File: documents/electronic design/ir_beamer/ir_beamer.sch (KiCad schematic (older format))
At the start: 10 parts, among them U1 74HC595D, U2 STM32F103HEADER

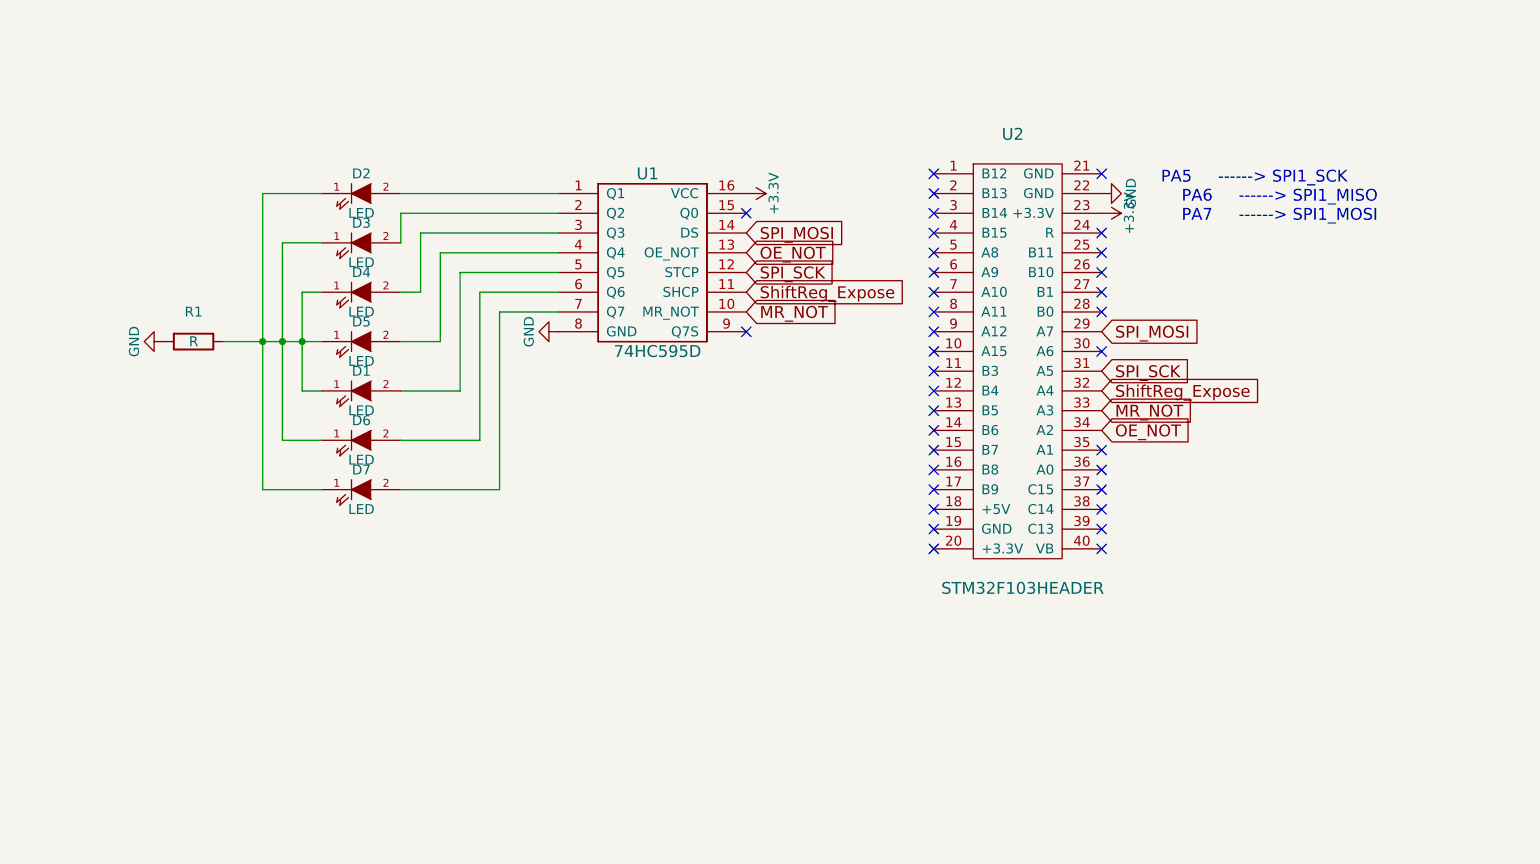
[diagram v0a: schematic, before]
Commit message: update pcb
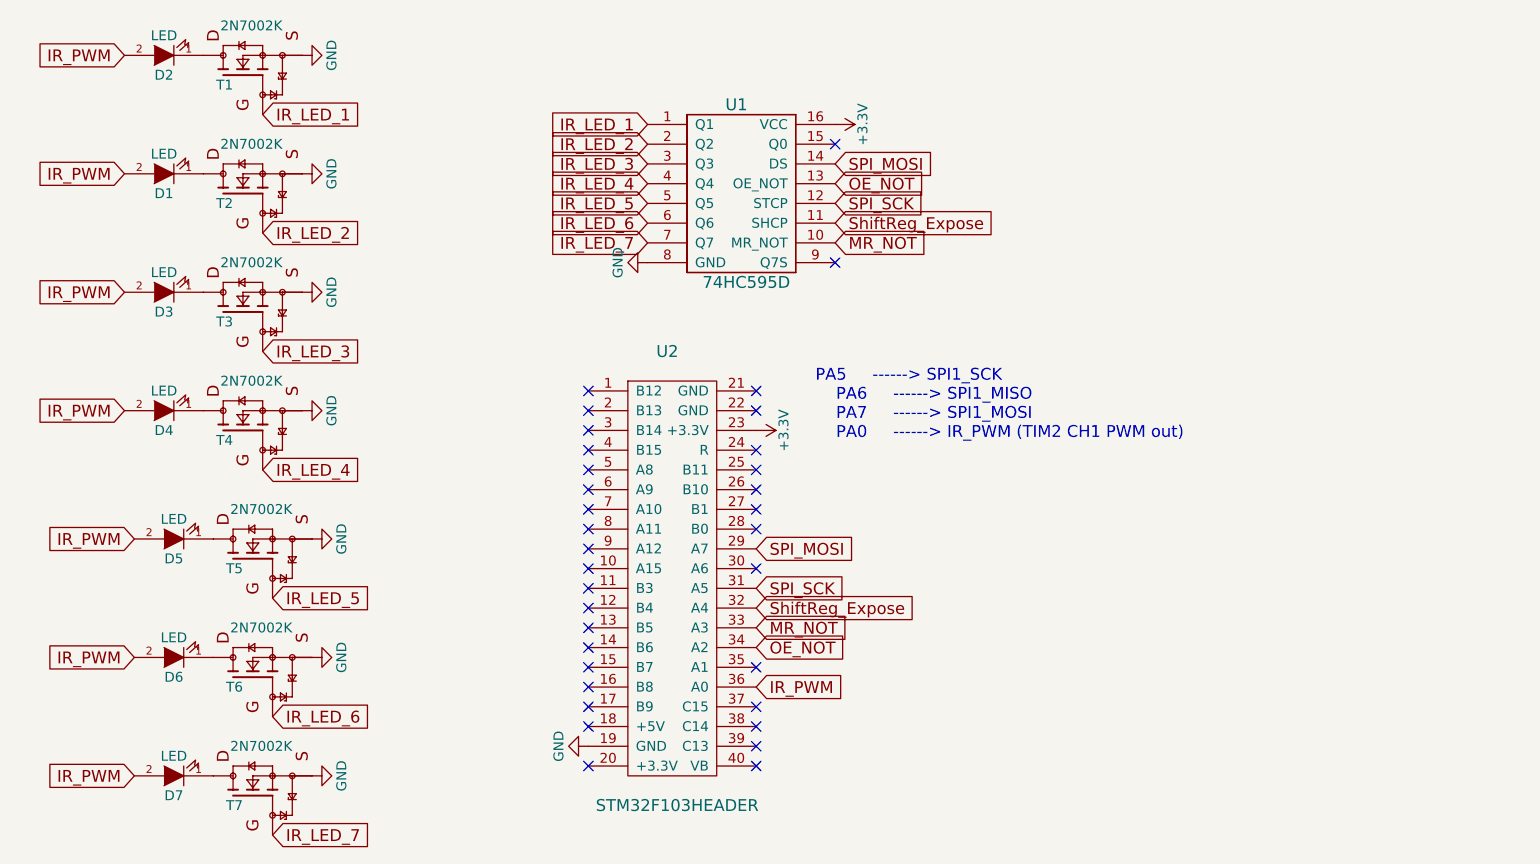
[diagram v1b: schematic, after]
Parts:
- removed R1: R, Resistors_SMD:R_0805_HandSoldering, symbol R
- added T1, T2, T3, T4, T5, T6, T7: 2N7002K, footprints:SOT23, symbol 2N7002K
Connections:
- net GND: now also U2.19 (GND), T1.2 (S), T2.2 (S), T3.2 (S), T4.2 (S), T5.2 (S), T6.2 (S), T7.2 (S); no longer U2.22 (GND)
- net IR_LED_5: now reaches U1.5 (Q5)
- net IR_LED_5: now also T5.1 (G); no longer D1.2 (A)
- net IR_LED_6: now reaches U1.6 (Q6)
- net IR_LED_6: now also T6.1 (G); no longer D6.2 (A)
- net IR_LED_7: now reaches U1.7 (Q7)
- net IR_LED_7: now also T7.1 (G); no longer D7.2 (A)
- net IR_LED_1: now reaches U1.1 (Q1)
- net IR_LED_1: now also T1.1 (G); no longer D2.2 (A)
- net IR_LED_2: now reaches U1.2 (Q2)
- net IR_LED_2: now also T2.1 (G); no longer D3.2 (A)
- net IR_LED_3: now reaches U1.3 (Q3)
- net IR_LED_3: now also T3.1 (G); no longer D4.2 (A)
- net IR_LED_4: now reaches U1.4 (Q4)
- net IR_LED_4: now also T4.1 (G); no longer D5.2 (A)
- net IR_PWM: now reaches U2.36 (A0)
- net IR_PWM: now also D1.2 (A), D2.2 (A), D3.2 (A), D4.2 (A), D5.2 (A), D6.2 (A), D7.2 (A)
- new net: D2.1 (K), T1.3 (D)
- new net: D1.1 (K), T2.3 (D)
- new net: D3.1 (K), T3.3 (D)
- new net: D4.1 (K), T4.3 (D)
- new net: D5.1 (K), T5.3 (D)
- new net: D6.1 (K), T6.3 (D)
- new net: D7.1 (K), T7.3 (D)
- no-connect marks 35 -> 34
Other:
- note added: "PA5 ------> SPI1_SCK\n PA6 ------> SPI1_MISO\n PA7 ------> SPI1_MOSI\n PA0 ------> IR_PWM (TIM2 CH1 PWM out)"
- note removed: "PA5 ------> SPI1_SCK\n PA6 ------> SPI1_MISO\n PA7 ------> SPI1_MOSI"
- moved on the sheet: D2, U1
